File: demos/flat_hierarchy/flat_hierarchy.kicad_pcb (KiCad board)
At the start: 2 copper layers, 160 x 99.1 mm, 64 parts, among them J1 DB9-FEMAL, P1 CONN_2, P2 SUPP28, P3 SUPP40, Q1 BC237, Q2 BC307, Q3 BC307, U1 24Cxx, U2 74HC125, U3 7805, U4 LT1373, U5 PIC_18_PINS, U6 PIC_8_PINS

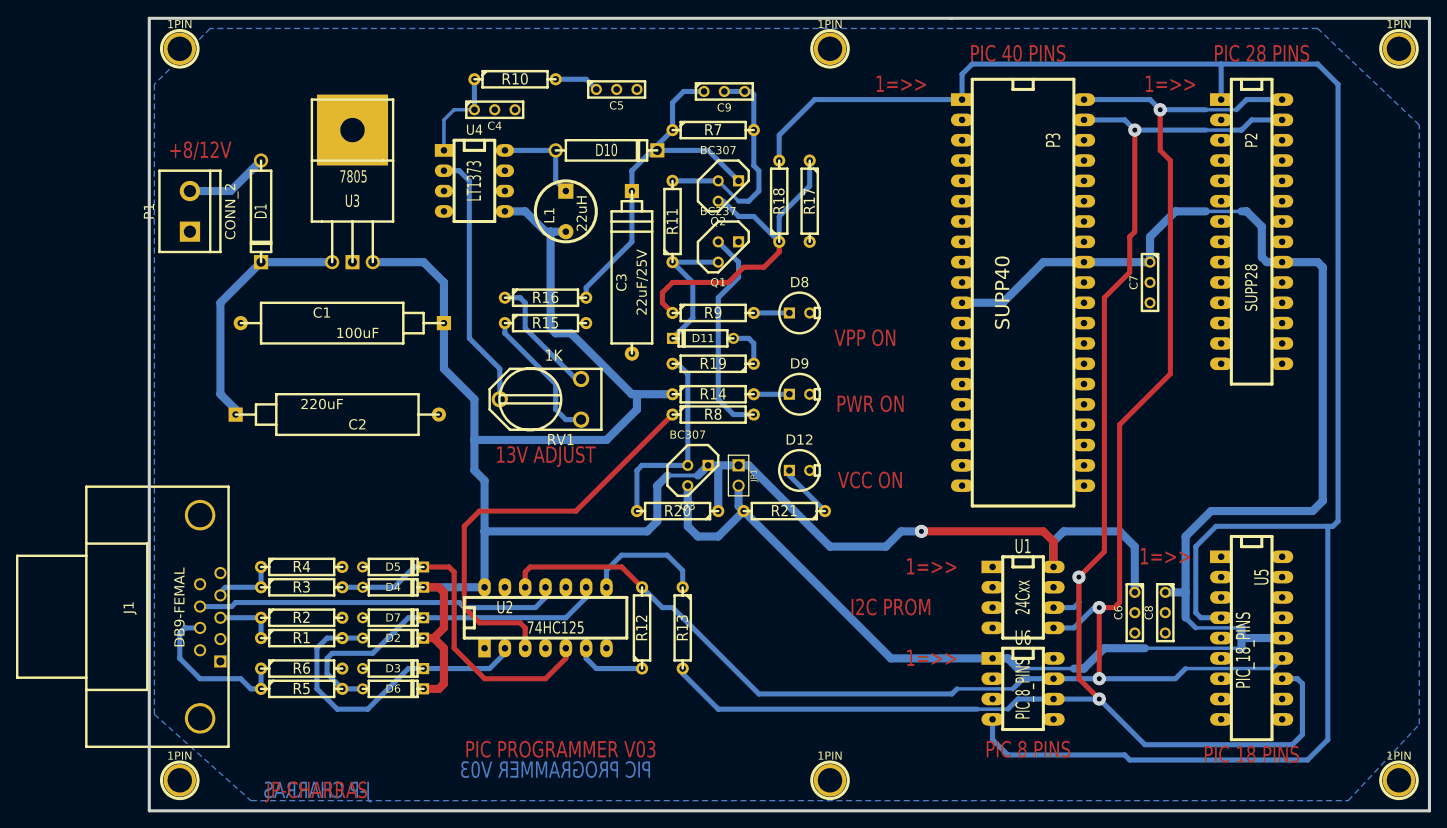
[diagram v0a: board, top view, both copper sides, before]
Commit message: Update demo files
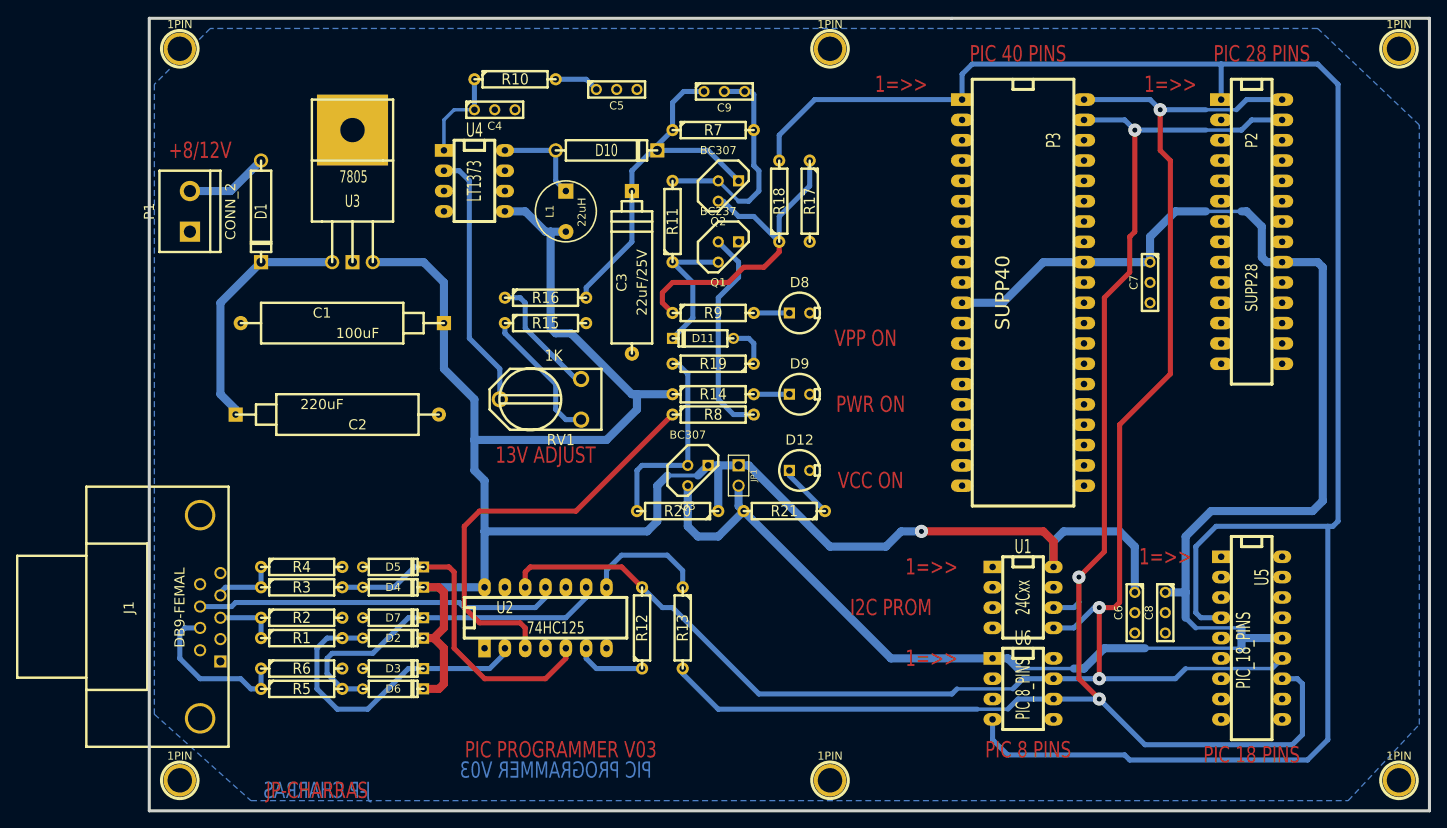
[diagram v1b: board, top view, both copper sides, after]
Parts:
- C1, C2: footprint CP10 -> discret:CP10
- C3: footprint CP8 -> discret:CP8
- C4, C5, C6, C7, C8, C9: footprint C1-1 -> discret:C1-1
- D1, D10: footprint D5 -> discret:D5
- D11, D2, D3, D4, D5, D6, D7: footprint D3 -> discret:D3
- D12, D8, D9: footprint LEDV -> discret:LEDV
- J1: footprint DB9FC -> connect:DB9FC
- JP1: footprint PIN_ARRAY_2X1 -> pin_array:PIN_ARRAY_2X1
- L1: footprint INDUCTOR_V -> inductors:INDUCTOR_V
- P1: footprint bornier2 -> connect:bornier2
- Q1, Q2, Q3: footprint TO92 -> discret:TO92
- R1, R10, R11, R12, R13, R14, R15, R16, R17, R18, R19, R2, R20, R21, R3, R4, R5, R6, R7, R8, R9: footprint R4 -> discret:R4
- RV1: footprint RV2X4 -> discret:RV2X4
- U1, U4, U6: footprint 8DIP-ELL300 -> dip_sockets:DIP-8__300_ELL
- U2: footprint 14DIP-ELL300 -> dip_sockets:DIP-14__300_ELL
- U3: footprint LM78XX -> discret:LM78XX
- U5: footprint 18DIP-ELL300 -> dip_sockets:DIP-18__300_ELL
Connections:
- net /pic_programmer/PC-DATA-OUT renamed /pic_programmer/DTR
- net /pic_programmer/RTS renamed /pic_programmer/PC-CLOCK-OUT
- net /sockets/CLOCK-RB6 renamed CLOCK-RB6
- net /sockets/DATA-RB7 renamed DATA-RB7
- net /sockets/VCC_PIC renamed VCC_PIC
- P2 pad 1: /sockets/VPP-MCLR -> VPP-MCLR
- P3 pad 1: /sockets/VPP-MCLR -> VPP-MCLR
- R18 pad 2: N-000030 -> VPP-MCLR
- U5 pad 4: /sockets/VPP-MCLR -> VPP-MCLR
- U6 pad 4: /sockets/VPP-MCLR -> VPP-MCLR
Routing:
- net VPP-MCLR: track 0.00 -> 242.7 mm
- net /sockets/VPP-MCLR: track 239.5 -> 0.00 mm
- net N-000030: track 3.18 -> 0.00 mm
